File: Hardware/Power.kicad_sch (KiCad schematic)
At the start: 40 parts, among them J2 JST_2mm_LiPo, Q2 SIL2308, U10 MCP73833_MSOP, U11 AP2112K-3.3, U12 STLQ015-3.3, U4 MAX17048, U5 AP2112K-3.3

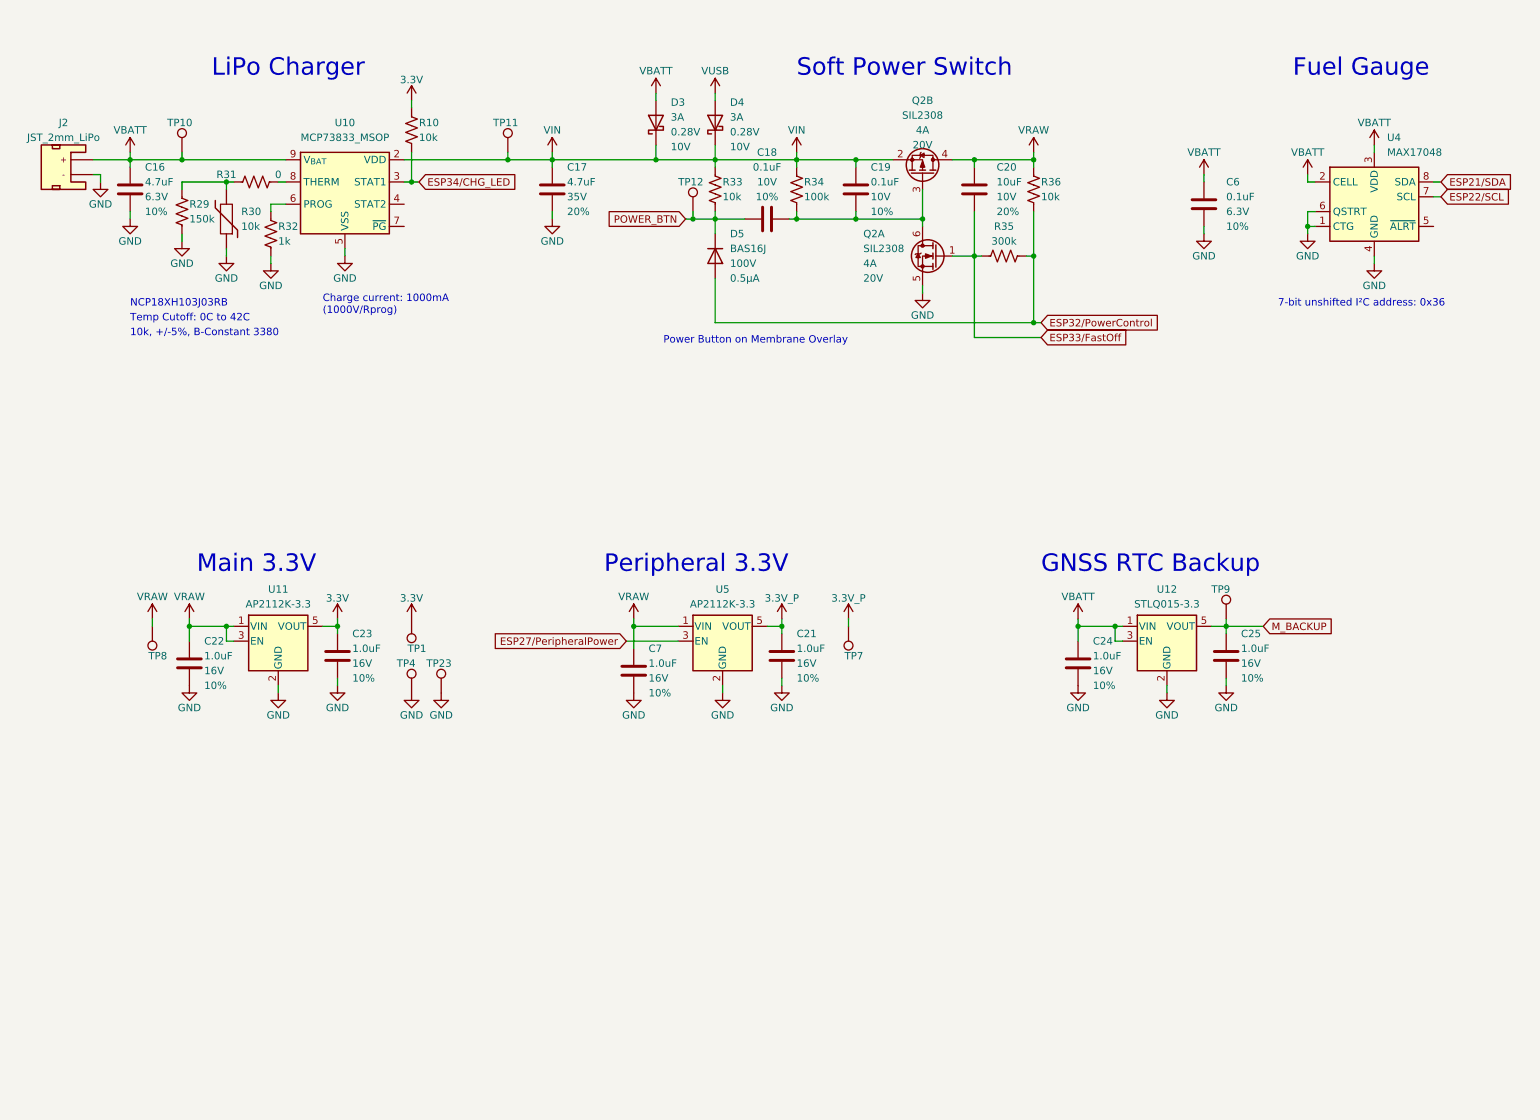
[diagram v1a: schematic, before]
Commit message: v1.1 routed
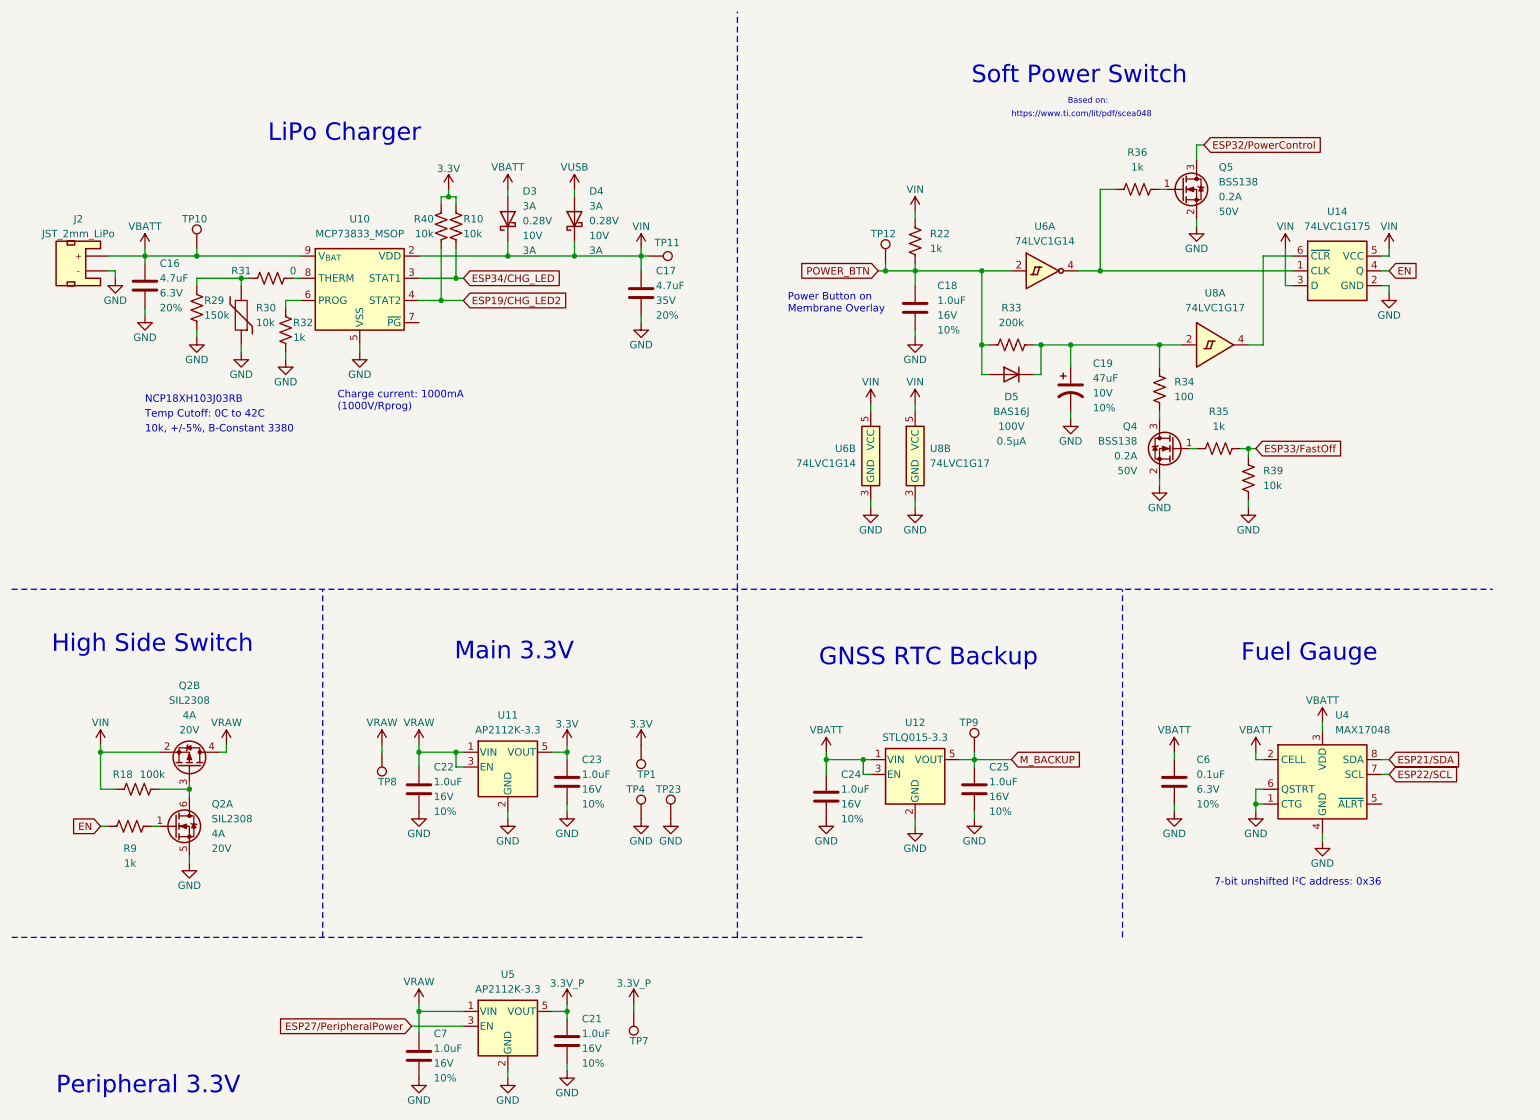
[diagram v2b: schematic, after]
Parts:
- removed C18, C19: 0.1uF, SparkFun-Capacitor:C_0402_1005Metric, symbol SparkFun-Capacitor:0.1uF_0402_10V_10%
- removed C20: 10uF, SparkFun-Capacitor:C_0603_1608Metric, symbol SparkFun-Capacitor:10uF_0603_10V_20%
- removed R33, R36: 10k, SparkFun-Resistor:R_0402_1005Metric, symbol SparkFun-Resistor:10k_0402
- removed R34: 100k, SparkFun-Resistor:R_0402_1005Metric, symbol SparkFun-Resistor:100k_0402
- removed R35: 300k, SparkFun-Resistor:R_0603_1608Metric, symbol SparkFun-Resistor:300k_0603
- added C18: 1.0uF, SparkFun-Capacitor:C_0402_1005Metric, symbol SparkFun-Capacitor:1.0uF_0402_16V_10%
- added C19: 47uF, SparkFun-Capacitor:EIA-3528, symbol SparkFun-Capacitor:47uF_3528_10V_10%
- added Q4, Q5: BSS138, SparkFun-Semiconductor-Standard:SOT23-3, symbol SparkFun-DiscreteSemi:Q_NMOS_0.2A_50V
- added R18: 100k, SparkFun-Resistor:R_0402_1005Metric, symbol SparkFun-Resistor:100k_0402
- added R22, R35, R36, R9: 1k, SparkFun-Resistor:R_0402_1005Metric, symbol SparkFun-Resistor:1k_0402
- added R33: 200k, SparkFun-Resistor:R_0402_1005Metric, symbol SparkFun-Resistor:200k_0402
- added R34: 100, SparkFun-Resistor:R_0402_1005Metric, symbol SparkFun-Resistor:100_0402
- added R39, R40: 10k, SparkFun-Resistor:R_0402_1005Metric, symbol SparkFun-Resistor:10k_0402
- added U14: 74LVC1G175, SparkFun-Semiconductor-Standard:SOT-323, symbol SparkFun-IC-Logic:74LVC1G175
- added U6: 74LVC1G14, SparkFun-Semiconductor-Standard:SOT-353, symbol SparkFun-IC-Logic:74LVC1G14
- added U8: 74LVC1G17, SparkFun-Semiconductor-Standard:SOT-353, symbol SparkFun-IC-Logic:74LVC1G17
- C16: Tolerance 10% -> 20%
- D3, D4: IMax (none) -> 3A
- J2: footprint SparkFun-Connector:JST-2-SMD -> SparkFun-Connector:JST_SMD_2.0mm-2
- TP1, TP10, TP11, TP12, TP23, TP4, TP7, TP8, TP9: footprint SparkFun-Connector:1X01 -> SparkFun-Connector:1x01
- U10: footprint SparkFun-Semiconductor-Standard:MSOP10 -> SparkFun-Semiconductor-Standard:MSOP-10
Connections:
- net 3.3V: now also R40.1
- net ESP32/PowerControl: now also Q5.3 (D); no longer D5.A
- net ESP33/FastOff: now also R35.2, R39.1; no longer Q2.1 (G)
- net GND: now also C18.2, C19.2, Q4.2 (S), Q5.2 (S), R39.2, U14.2 (GND), U6.3 (GND), U8.3 (GND)
- net POWER_BTN: now also D5.A, C18.1, R22.2, R33.2, U6.2; no longer D5.C
- net VDD: now also R18.2, R22.1, U14.3 (D), U14.5 (VCC), U6.5 (VCC), U8.5 (VCC)
- net at Q2.3 (G), Q2.6 (D): now also R18.1
- net ESP19/CHG_LED2: now reaches U10.4 (STAT2)
- net ESP19/CHG_LED2: now also R40.2
- new net: Q2.1 (G), R9.1
- new net: R36.1, U14.1 (CLK), U6.4
- new net: U14.6 (~{CLR}), U8.4
- new net: Q4.1 (G), R35.1
- new net: C19.1, D5.C, R33.1, R34.1, U8.2
- new net: Q5.1 (G), R36.2
- new net: Q4.3 (D), R34.2
- new net EN: R9.2, U14.4 (Q)
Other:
- note added: "Based on:"
- note added: "High Side Switch"
- note added: "https://www.ti.com/lit/pdf/scea048"
- moved on the sheet: C16, C17, C21, C22, C23, C24, C25, C6, C7, D3, D4, J2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

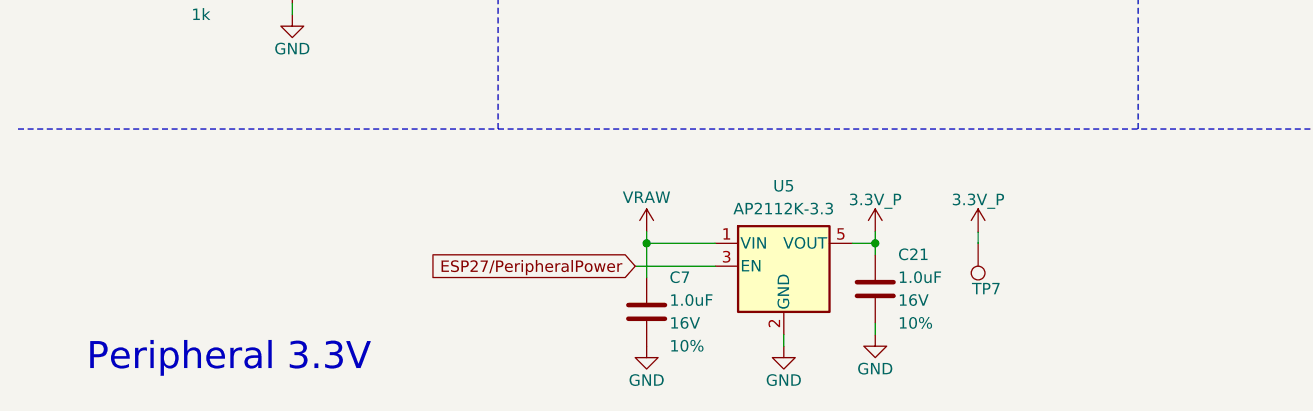
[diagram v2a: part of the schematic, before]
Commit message: V1.1 Panelized
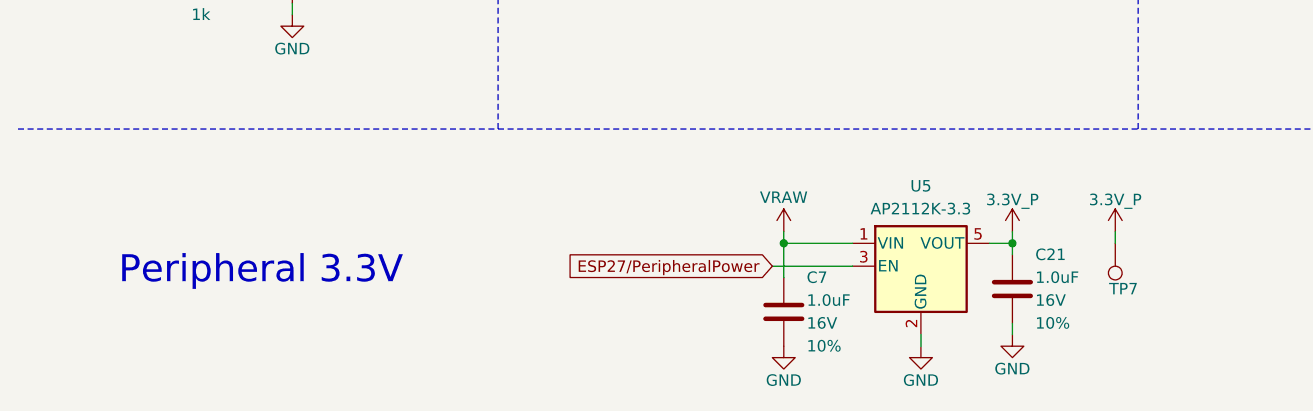
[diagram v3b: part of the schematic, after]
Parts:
- R34: footprint SparkFun-Resistor:R_0402_1005Metric -> SparkFun-Resistor:R_0603_1608Metric; symbol SparkFun-Resistor:100_0402 -> SparkFun-Resistor:100_0603; PROD_ID RES-14962 -> RES-07863
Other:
- moved on the sheet: C21, C7, TP7, U5
